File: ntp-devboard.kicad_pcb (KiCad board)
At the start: 2 copper layers, 42.4 x 51 mm, 74 parts, among them J1 USB_C_Receptacle_USB2.0_14P, J2 Conn_01x07, J3 Conn_01x20, J4 Conn_01x04, J5 Conn_01x02, J6 RJ45_Hanrun_HR911105A_Horizon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, SW1 SW_Push, U1 RP2040, U2 MCP1700x-330xxTT, U3 LAN9250/ML, U4 W25Q16JVUXIQ TR, Y1 12 MHz, Y2 25 MHz

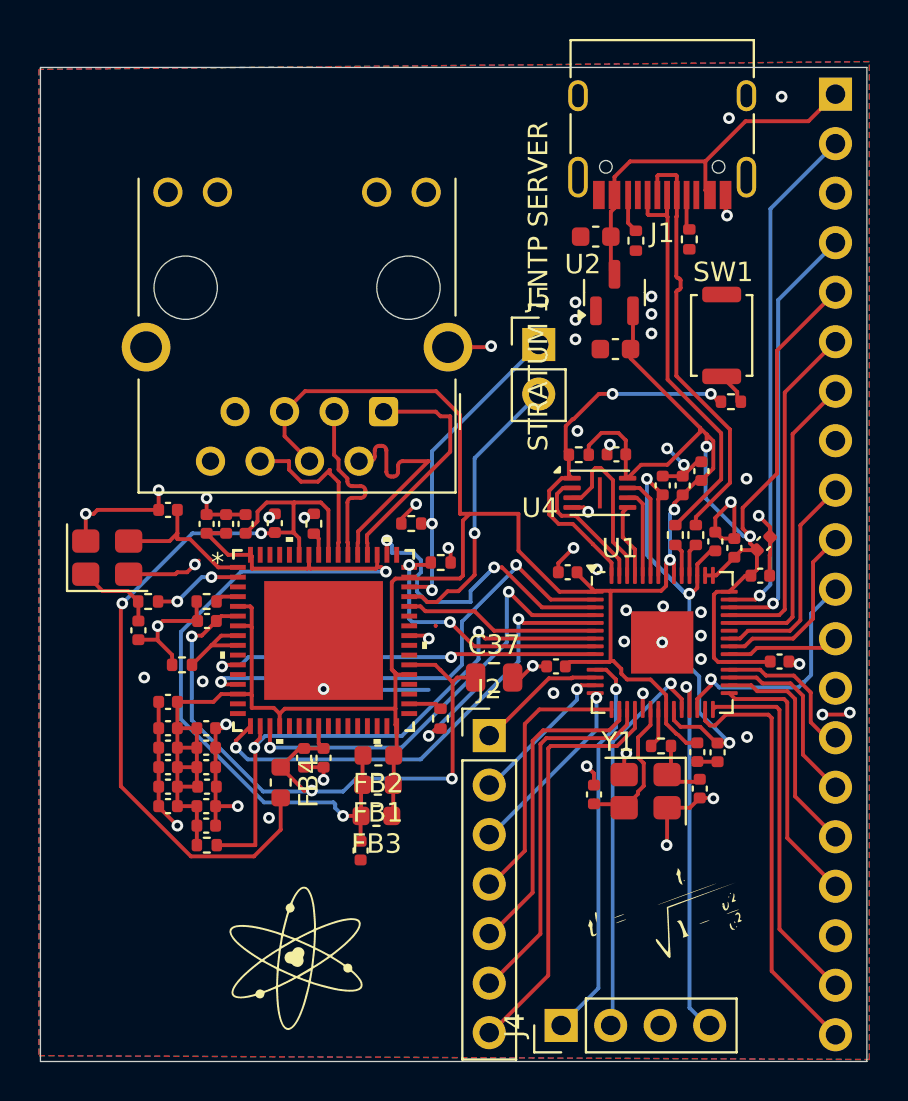
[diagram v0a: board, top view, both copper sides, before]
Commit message: cooked ah decoupling caps
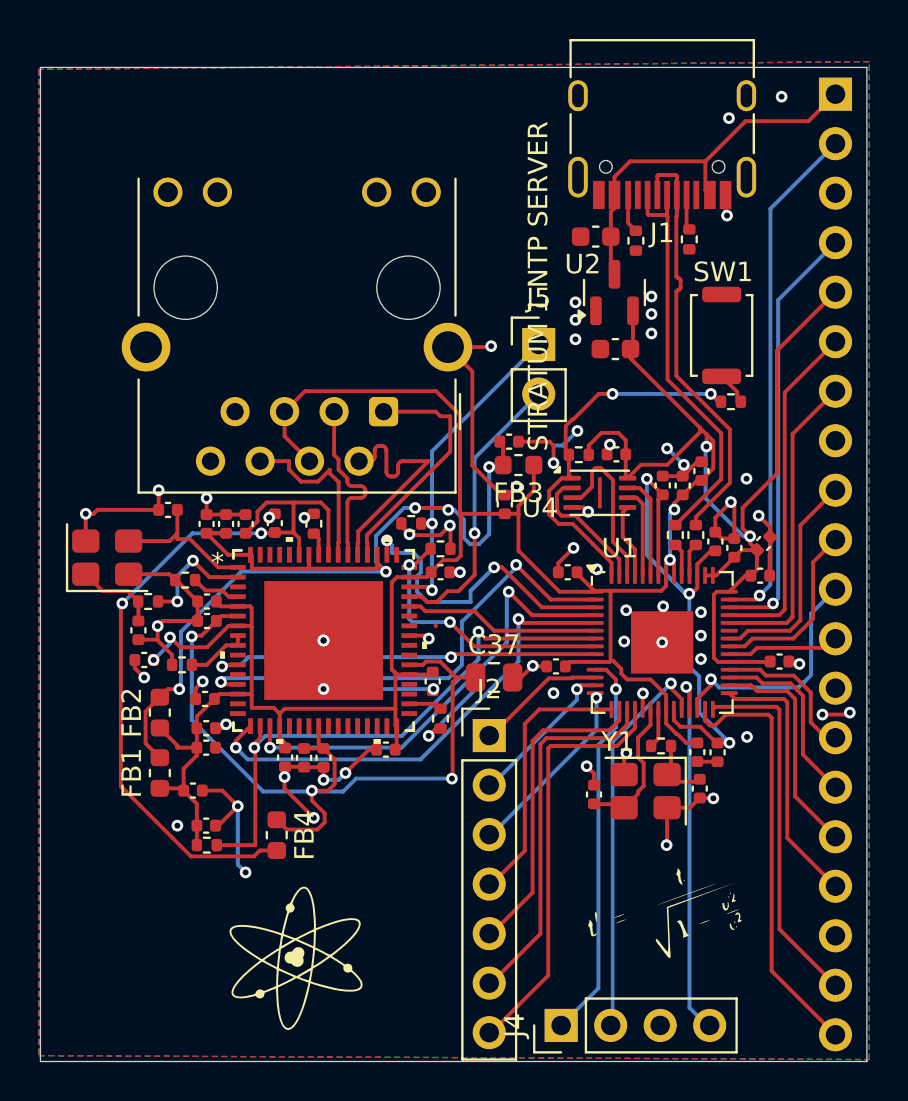
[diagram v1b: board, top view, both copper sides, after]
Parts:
- C18, C19: value 33pF -> 15pF
- R15: value 12.1K -> 12K
- R3, R4: value 27 -> 22
- moved C24 23.2 mm to (145.3, 104.5), turned to 90 degrees
- moved C38 22.3 mm to (145.5, 101.3), turned to 0 degrees
- moved FB3 19.4 mm to (146.0, 102.5)
- moved C26 17.2 mm to (142.0, 108.0), turned to 0 degrees
- moved C27 14.0 mm to (141.6, 113.6), turned to -90 degrees
- moved FB2 11.4 mm to (127.6, 115.2), turned to 90 degrees
- moved FB1 11.2 mm to (127.6, 118.3), turned to 90 degrees
- moved C25 9.71 mm to (130.0, 109.5)
- moved C32 9.26 mm to (139.2, 117.1), turned to 180 degrees
- moved C33 7.25 mm to (126.8, 112.5), turned to 180 degrees
- moved C28 6.19 mm to (134.0, 117.5), turned to -90 degrees
- moved FB4 2.71 mm to (133.6, 121.5)
- moved C29 1.91 mm to (129.9, 114.5)
- moved R16 1.56 mm to (128.9, 108.4)
- moved C21 1.05 mm to (129.3, 119.2)
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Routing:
- net GND: track 80.5 -> 102.3 mm, vias 57 -> 65
- net C34: track 37.0 -> 42.3 mm
- net C40: track 45.6 -> 48.5 mm, vias 2 -> 5
- net +3V3: track 163.3 -> 165.9 mm, vias 4 -> 6
- net C35: track 42.1 -> 39.8 mm
- net OSOUT: track 4.61 -> 6.08 mm
- net Net-(U3-OSCVSS): track 1.20 -> 2.55 mm
- net Net-(U3-FXLOSEN): track 4.33 -> 3.27 mm
